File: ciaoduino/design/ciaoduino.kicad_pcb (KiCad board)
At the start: 2 copper layers, 50.5 x 47.8 mm, 19 parts, among them P1 ICSP, P2 CONN_01X02, P3 USB_OTG, P4 CONN_01X06, P5 CONN_01X06, P6 CONN_01X04, P7 CONN_01X14, SW1 SW_PUSH, SW2 SW_PUSH, U2 ATmega32U4-AU, X1 CRYSTAL_SMD

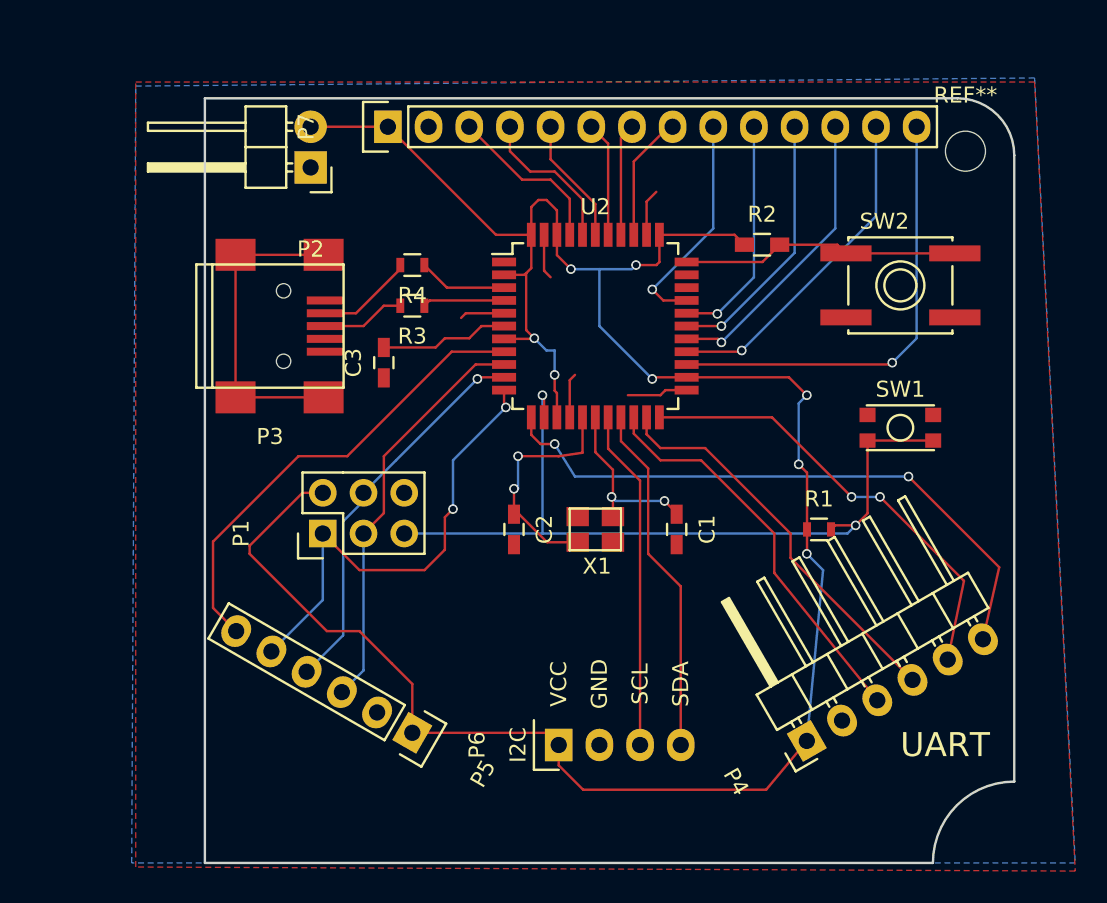
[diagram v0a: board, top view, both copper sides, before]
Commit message: Rework layout.
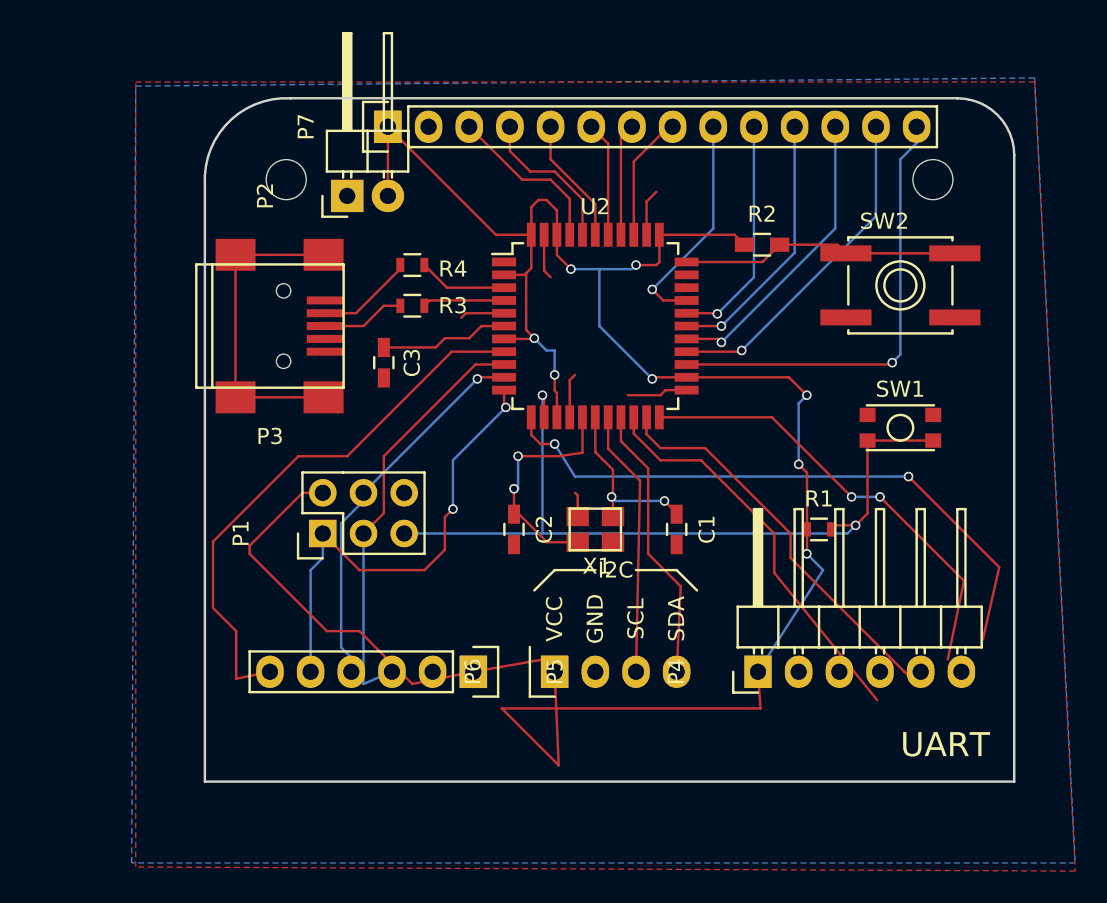
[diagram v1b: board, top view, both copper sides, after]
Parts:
- added REF**: MountingHole_2.5mm, Mounting_Holes:MountingHole_2.5mm, F.Cu at (131.8, 65.8)
- moved P5 5.39 mm to (143.5, 96.5), turned to 270 degrees
- moved P4 5.29 mm to (161.3, 96.5), turned to 90 degrees
- moved P6 4.58 mm to (148.6, 96.5)
- moved P2 2.90 mm to (135.6, 66.8), turned to 90 degrees
- moved REF** 2.70 mm to (172.2, 65.8)
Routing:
- net usart_tx: track 24.9 -> 5.07 mm
- net usart_cts: track 28.3 -> 48.1 mm
- net SCLK: track 25.7 -> 31.2 mm
- net SS: track 29.3 -> 34.4 mm
- net SCL: track 21.3 -> 16.7 mm
- net SDA: track 22.0 -> 17.4 mm
- net GND: track 15.1 -> 16.7 mm
- net VCC: track 145.5 -> 144.5 mm
- net MOSI: track 24.4 -> 23.8 mm
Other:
- board size 50.5 x 47.8 mm -> 50.5 x 42.7 mm

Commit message: Rework layout.
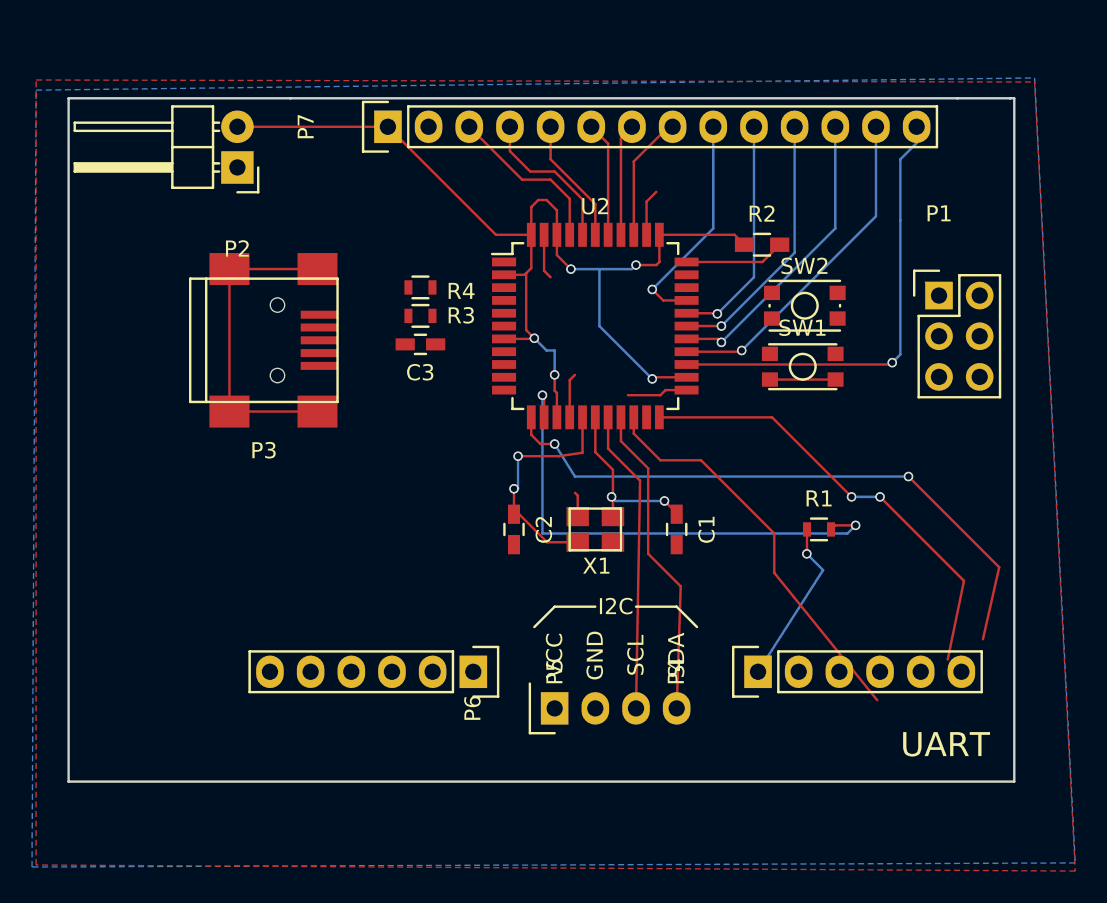
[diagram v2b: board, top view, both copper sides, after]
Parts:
- removed REF** (x2): MountingHole_2.5mm, Mounting_Holes:MountingHole_2.5mm
- P4: footprint Pin_Headers:Pin_Header_Angled_1x06 -> Pin_Headers:Pin_Header_Straight_1x06
- SW2: footprint Buttons_Switches_SMD:SW_SPST_EVQP0 -> Buttons_Switches_SMD:SW_SPST_KMR2
- moved P1 41.3 mm to (172.6, 73.0), turned to 0 degrees
- moved SW1 7.19 mm to (164.1, 77.5)
- moved P2 7.08 mm to (128.8, 65.0), turned to 180 degrees
- moved SW2 6.10 mm to (164.2, 73.7)
- moved C3 2.56 mm to (140.2, 76.1), turned to 0 degrees
- moved P6 2.29 mm to (148.6, 98.8)
- moved R4 1.49 mm to (140.2, 72.5)
- moved P3 0.97 mm to (130.4, 75.8)
- moved R3 0.81 mm to (140.2, 74.3)
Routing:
- net VCC: track 144.5 -> 79.9 mm, vias 8 -> 6
- net SS: track 34.4 -> 0.00 mm
- net SCLK: track 31.2 -> 0.64 mm
- net MISO: track 29.6 -> 1.30 mm, vias 2 -> 0
- net MOSI: track 23.8 -> 1.52 mm, vias 1 -> 0
- net usart_cts: track 48.1 -> 28.3 mm
- net RESET: track 49.8 -> 35.6 mm
- net Net-(R2-Pad2): track 17.4 -> 6.26 mm
- net Net-(C3-Pad2): track 8.06 -> 0.00 mm
- net Net-(P3-Pad2): track 6.08 -> 0.24 mm
- net Net-(R4-Pad1): track 5.56 -> 0.00 mm
- net Net-(P3-Pad3): track 5.22 -> 0.00 mm
- net Net-(R3-Pad1): track 5.12 -> 0.00 mm
- net usart_tx: track 5.07 -> 0.00 mm
- net GND: track 16.7 -> 13.9 mm
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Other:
- board size 50.5 x 42.7 mm -> 59.1 x 42.7 mm
